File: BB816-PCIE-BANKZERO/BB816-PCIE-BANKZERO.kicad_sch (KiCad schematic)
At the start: 22 parts, among them J1 Bypass, U1 AS7C256B-15PIN, U10 74HC138, U11 W65C51NxP, U12 W65C51NxP, U15 74HC32, U16 74HC138, U2 AS7C256B-15PIN, U23 74HC04, U3 AT28C256-15PU, U4 74HC138, U5 74HC148, U6 74HC125, U7 74HC283, U8 W65C22SxP, U9 74HC32

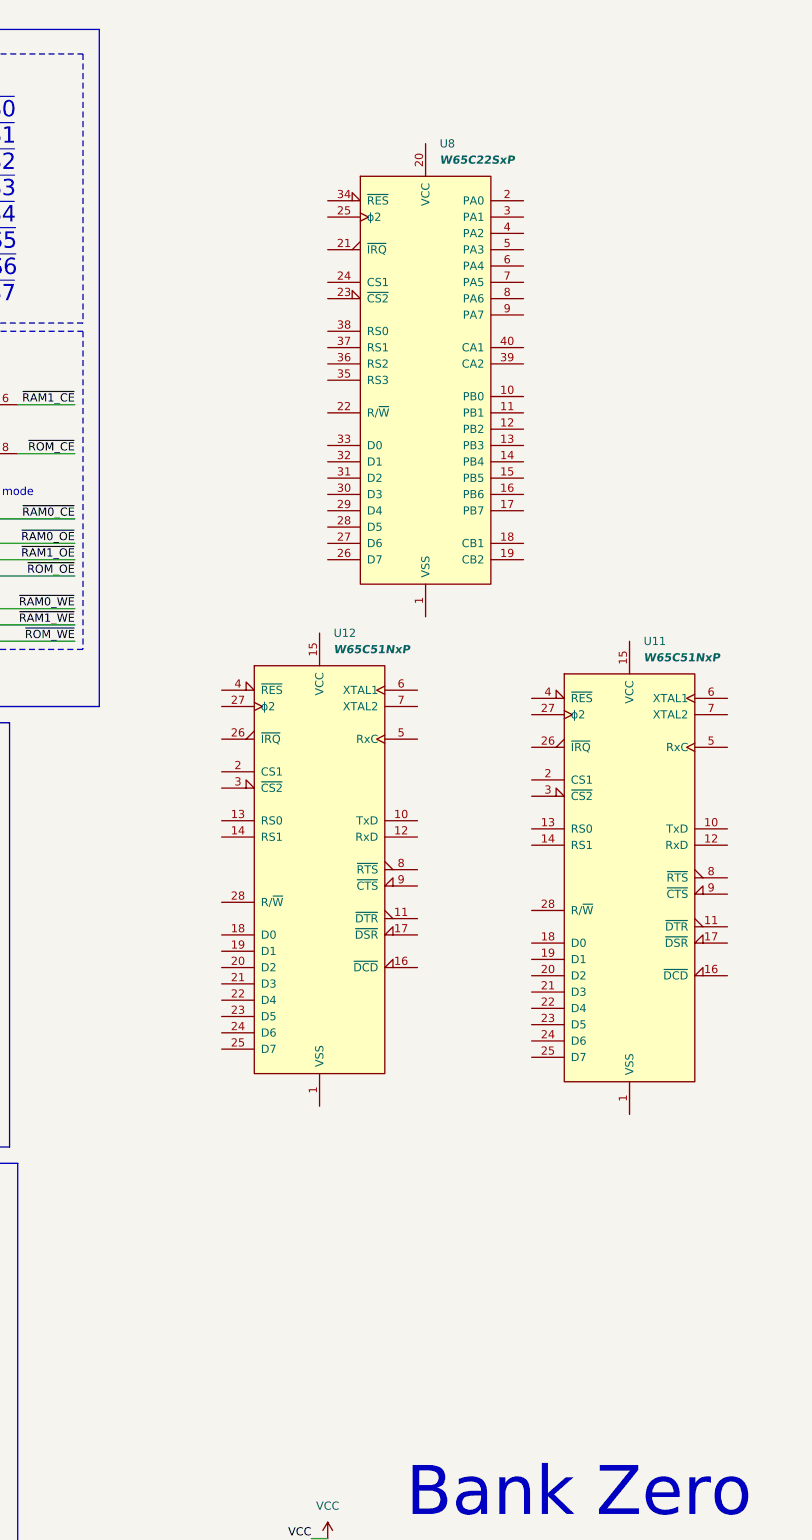
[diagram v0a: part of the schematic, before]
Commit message: VIA
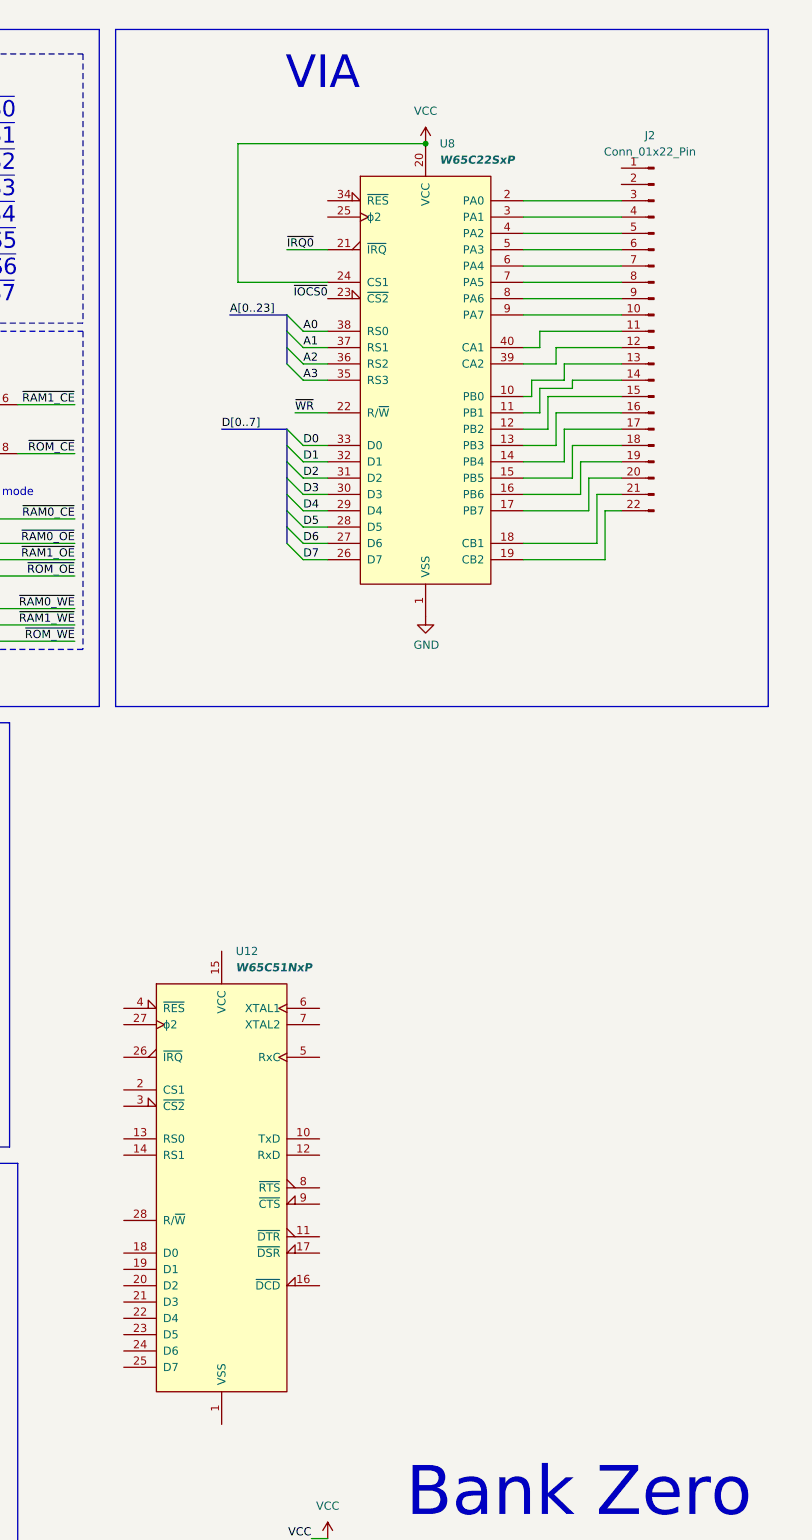
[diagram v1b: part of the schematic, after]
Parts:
- removed U11: W65C51NxP, Package_DIP:DIP-28_W15.24mm_Socket, symbol BB816-MATX-PCIE:W65C51NxP
- added J2: Conn_01x22_Pin, Connector_PinHeader_2.54mm:PinHeader_1x22_P2.54mm_Horizontal, symbol Connector:Conn_01x22_Pin
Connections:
- net A0: now also U8.38 (RS0)
- net A1: now also U8.37 (RS1)
- net A2: now also U8.36 (RS2)
- net A3: now also U8.35 (RS3)
- net D0: now also U8.33 (D0)
- net D1: now also U8.32 (D1)
- net D2: now also U8.31 (D2)
- net D3: now also U8.30 (D3)
- net D4: now also U8.29 (D4)
- net D5: now also U8.28 (D5)
- net D6: now also U8.27 (D6)
- net D7: now also U8.26 (D7)
- net GND: now also U8.1 (VSS)
- net VCC: now also U8.20 (VCC), U8.24 (CS1)
- net ~{IOCS0}: now also U8.23 (~{CS2})
- net ~{IRQ0}: now also U8.21 (~{IRQ})
- net ~{RAM0_WE}: now also U8.22 (R/~{W})
- net at U8.10 (PB0): now also J2.13 (Pin_13)
- net at U8.11 (PB1): now also J2.14 (Pin_14)
- net at U8.12 (PB2): now also J2.15 (Pin_15)
- net at U8.13 (PB3): now also J2.16 (Pin_16)
- net at U8.14 (PB4): now also J2.17 (Pin_17)
- net at U8.15 (PB5): now also J2.18 (Pin_18)
- net at U8.16 (PB6): now also J2.19 (Pin_19)
- net at U8.17 (PB7): now also J2.20 (Pin_20)
- net at U8.18 (CB1): now also J2.21 (Pin_21)
- net at U8.19 (CB2): now also J2.22 (Pin_22)
- net at U8.2 (PA0): now also J2.3 (Pin_3)
- net at U8.3 (PA1): now also J2.4 (Pin_4)
- net at U8.39 (CA2): now also J2.12 (Pin_12)
- net at U8.4 (PA2): now also J2.5 (Pin_5)
- net at U8.40 (CA1): now also J2.11 (Pin_11)
- net at U8.5 (PA3): now also J2.6 (Pin_6)
- net at U8.6 (PA4): now also J2.7 (Pin_7)
- net at U8.7 (PA5): now also J2.8 (Pin_8)
- net at U8.8 (PA6): now also J2.9 (Pin_9)
- net at U8.9 (PA7): now also J2.10 (Pin_10)
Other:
- note added: "VIA"
- moved on the sheet: U12
